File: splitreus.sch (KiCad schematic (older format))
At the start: 65 parts, among them J1 TRRS, SW0 SW_PUSH, SW1 SW_PUSH, SW10 SW_PUSH, SW11 SW_PUSH, SW12 SW_PUSH, SW13 SW_PUSH, SW14 SW_PUSH, SW15 SW_PUSH, SW16 SW_PUSH, SW17 SW_PUSH, SW18 SW_PUSH, SW19 SW_PUSH, SW2 SW_PUSH, SW20 SW_PUSH, SW21 SW_PUSH, SW22 SW_PUSH, SW23 SW_PUSH, SW24 SW_PUSH, SW25 SW_PUSH, SW26 SW_PUSH, SW27 SW_PUSH, SW28 SW_PUSH, SW29 SW_PUSH, SW3 SW_PUSH, SW30 SW_PUSH, SW4 SW_PUSH, SW5 SW_PUSH, SW6 SW_PUSH, SW7 SW_PUSH, SW8 SW_PUSH, SW9 SW_PUSH, U1 ProMicro

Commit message: a lot
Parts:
- D0, D1, D10, D11, D12, D13, D14, D15, D16, D17, D18, D19, D2, D20, D21, D22, D23, D24, D25, D26, D27, D28, D29, D3, D30, D4, D5, D6, D7, D8, D9: value DIODE_SCHOTTKY_SOT23 -> 1N4148; footprint keebio:Diode-Hybrid-reversible -> Custom Footies:Diode-Hybrid-reversible; symbol Keyboard_Parts:DIODE_SCHOTTKY_SOT23 -> pspice:DIODE
- RST1: footprint Connector_PinHeader_1.27mm:PinHeader_1x02_P1.27mm_Vertical -> Lily58-footprint:TACT_SWITCH_TVBP06
- SW0, SW1, SW10, SW11, SW12, SW13, SW14, SW15, SW16, SW17, SW18, SW19, SW2, SW20, SW21, SW22, SW23, SW24, SW25, SW26, SW27, SW28, SW29, SW3, SW30, SW4, SW5, SW6, SW7, SW8, SW9: footprint Custom Footies:MX-Alps-Choc-1U-No-reversible-fixed -> daprice_kail_mx:Kailh_socket_MX_reversible
- U1: footprint Lily58-footprint:ProMicro_rev2 -> Custom Footies:nice_nano
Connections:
- wire segments 149 -> 157
- no-connect marks 0 -> 3

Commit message: traces
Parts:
- added J2: battery, Connector_PinSocket_2.54mm:PinSocket_1x02_P2.54mm_Vertical, symbol Connector:Conn_01x02_Male
- SW0, SW1, SW10, SW11, SW12, SW13, SW14, SW15, SW16, SW17, SW18, SW19, SW2, SW20, SW21, SW22, SW23, SW24, SW25, SW26, SW27, SW28, SW29, SW3, SW30, SW4, SW5, SW6, SW7, SW8, SW9: footprint daprice_kail_mx:Kailh_socket_MX_reversible -> Custom Footies:Kailh_socket_MX_reversible_fix
- U1: symbol promicro:ProMicro -> promicro:nice_nano
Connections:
- net labels added: B+, B-

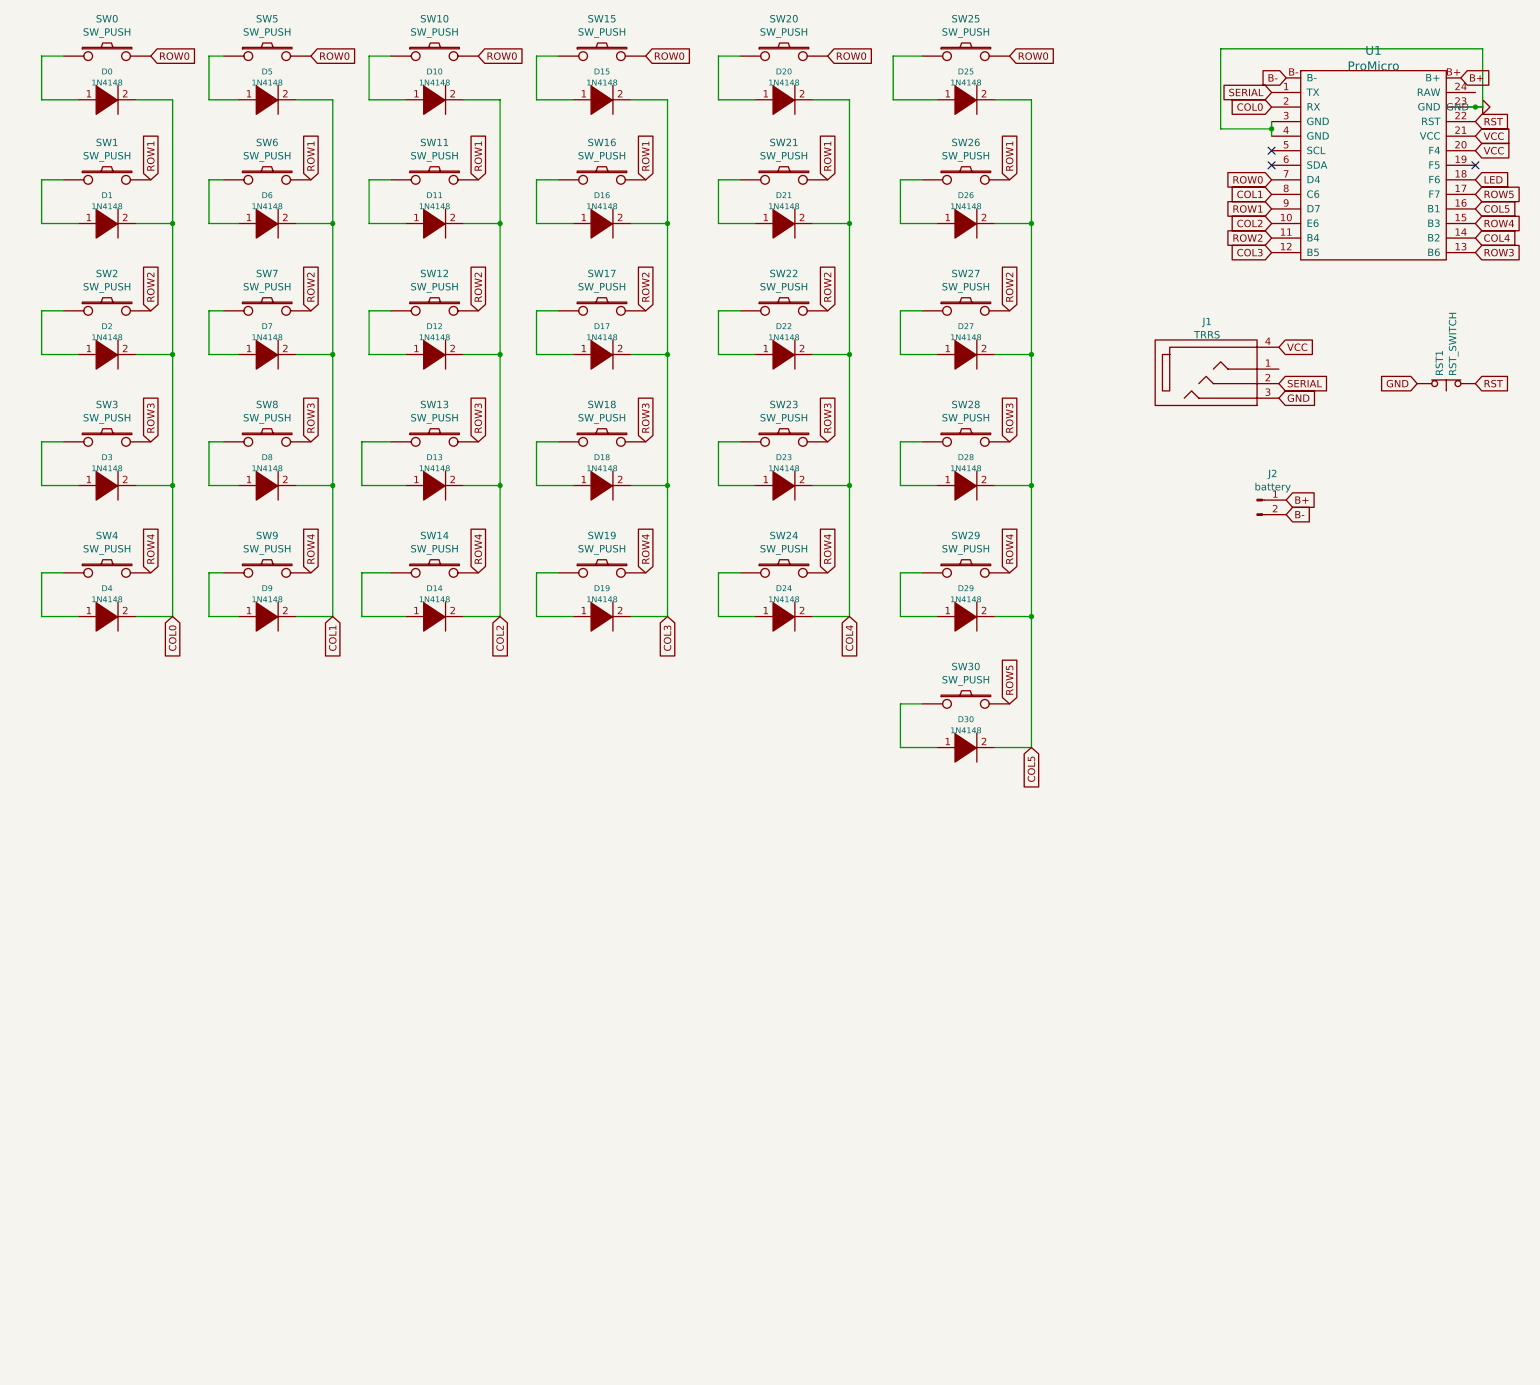
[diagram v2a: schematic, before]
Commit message: traces routed
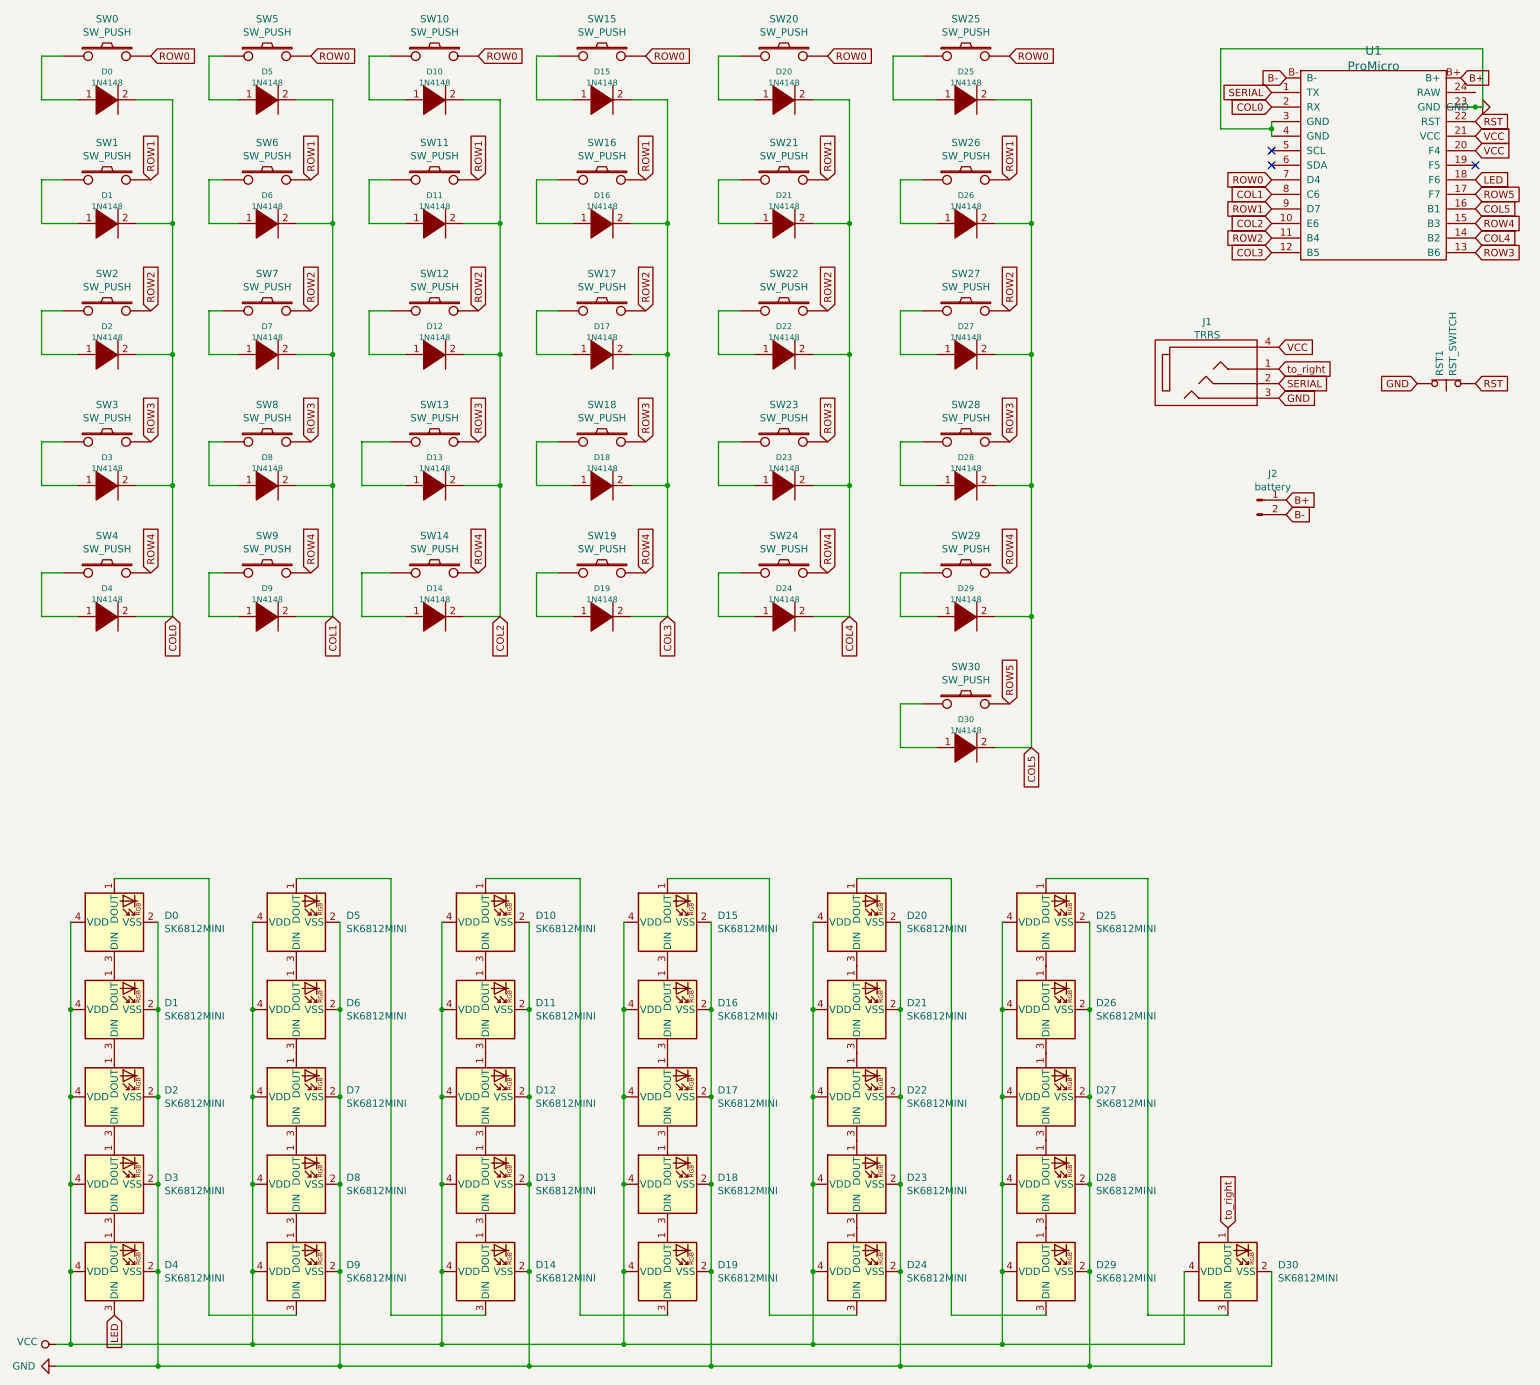
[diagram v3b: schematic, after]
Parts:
- added D0, D1, D10, D11, D12, D13, D14, D15, D16, D17, D18, D19, D2, D20, D21, D22, D23, D24, D25, D26, D27, D28, D29, D3, D30, D4, D5, D6, D7, D8, D9: SK6812MINI, LED_SMD:LED_SK6812MINI_PLCC4_3.5x3.5mm_P1.75mm, symbol LED:SK6812MINI
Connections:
- net GND: now also D0.2 (VSS), D1.2 (VSS), D10.2 (VSS), D11.2 (VSS), D12.2 (VSS), D13.2 (VSS), D14.2 (VSS), D15.2 (VSS), D16.2 (VSS), D17.2 (VSS), D18.2 (VSS), D19.2 (VSS), D2.2 (VSS), D20.2 (VSS), D21.2 (VSS), D22.2 (VSS), D23.2 (VSS), D24.2 (VSS), D25.2 (VSS), D26.2 (VSS), D27.2 (VSS), D28.2 (VSS), D29.2 (VSS), D3.2 (VSS), D30.2 (VSS), D4.2 (VSS), D5.2 (VSS), D6.2 (VSS), D7.2 (VSS), D8.2 (VSS), D9.2 (VSS)
- net LED: now also D4.3 (DIN)
- net VCC: now also D0.4 (VDD), D1.4 (VDD), D10.4 (VDD), D11.4 (VDD), D12.4 (VDD), D13.4 (VDD), D14.4 (VDD), D15.4 (VDD), D16.4 (VDD), D17.4 (VDD), D18.4 (VDD), D19.4 (VDD), D2.4 (VDD), D20.4 (VDD), D21.4 (VDD), D22.4 (VDD), D23.4 (VDD), D24.4 (VDD), D25.4 (VDD), D26.4 (VDD), D27.4 (VDD), D28.4 (VDD), D29.4 (VDD), D3.4 (VDD), D30.4 (VDD), D4.4 (VDD), D5.4 (VDD), D6.4 (VDD), D7.4 (VDD), D8.4 (VDD), D9.4 (VDD)
- net to_right: now reaches J1.1
- net to_right: now also D30.1 (DOUT)
- new net: D3.3 (DIN), D4.1 (DOUT)
- new net: D2.3 (DIN), D3.1 (DOUT)
- new net: D1.3 (DIN), D2.1 (DOUT)
- new net: D0.3 (DIN), D1.1 (DOUT)
- new net: D0.1 (DOUT), D9.3 (DIN)
- new net: D8.3 (DIN), D9.1 (DOUT)
- new net: D7.3 (DIN), D8.1 (DOUT)
- new net: D6.3 (DIN), D7.1 (DOUT)
- new net: D5.3 (DIN), D6.1 (DOUT)
- new net: D14.3 (DIN), D5.1 (DOUT)
- new net: D13.3 (DIN), D14.1 (DOUT)
- new net: D12.3 (DIN), D13.1 (DOUT)
- new net: D11.3 (DIN), D12.1 (DOUT)
- new net: D10.3 (DIN), D11.1 (DOUT)
- new net: D10.1 (DOUT), D19.3 (DIN)
- new net: D18.3 (DIN), D19.1 (DOUT)
- new net: D17.3 (DIN), D18.1 (DOUT)
- new net: D16.3 (DIN), D17.1 (DOUT)
- new net: D15.3 (DIN), D16.1 (DOUT)
- new net: D15.1 (DOUT), D24.3 (DIN)
- new net: D23.3 (DIN), D24.1 (DOUT)
- new net: D22.3 (DIN), D23.1 (DOUT)
- new net: D21.3 (DIN), D22.1 (DOUT)
- new net: D20.3 (DIN), D21.1 (DOUT)
- new net: D20.1 (DOUT), D29.3 (DIN)
- new net: D28.3 (DIN), D29.1 (DOUT)
- new net: D27.3 (DIN), D28.1 (DOUT)
- new net: D26.3 (DIN), D27.1 (DOUT)
- new net: D25.3 (DIN), D26.1 (DOUT)
- new net: D25.1 (DOUT), D30.3 (DIN)
